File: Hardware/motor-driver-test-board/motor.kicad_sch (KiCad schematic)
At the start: 8 parts, among them J1 Conn_01x11, J2 Conn_01x08, Q1 MMBF170, Q2 MMBF170, Q3 MMBF170, Q4 MMBF170, Q5 MMBF170, Q6 MMBF170

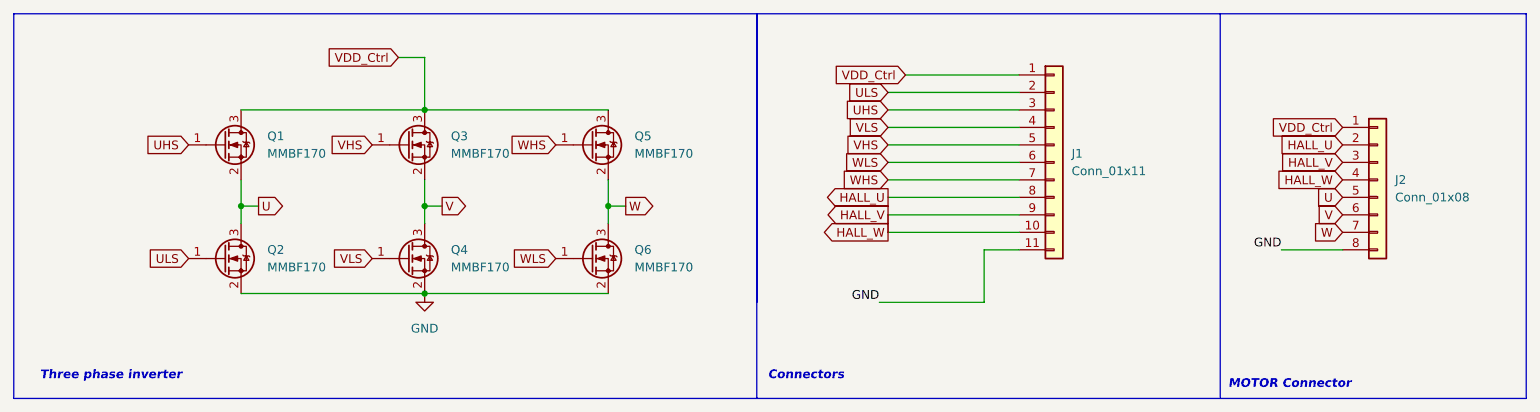
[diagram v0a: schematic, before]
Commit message: PCB REV 1.0
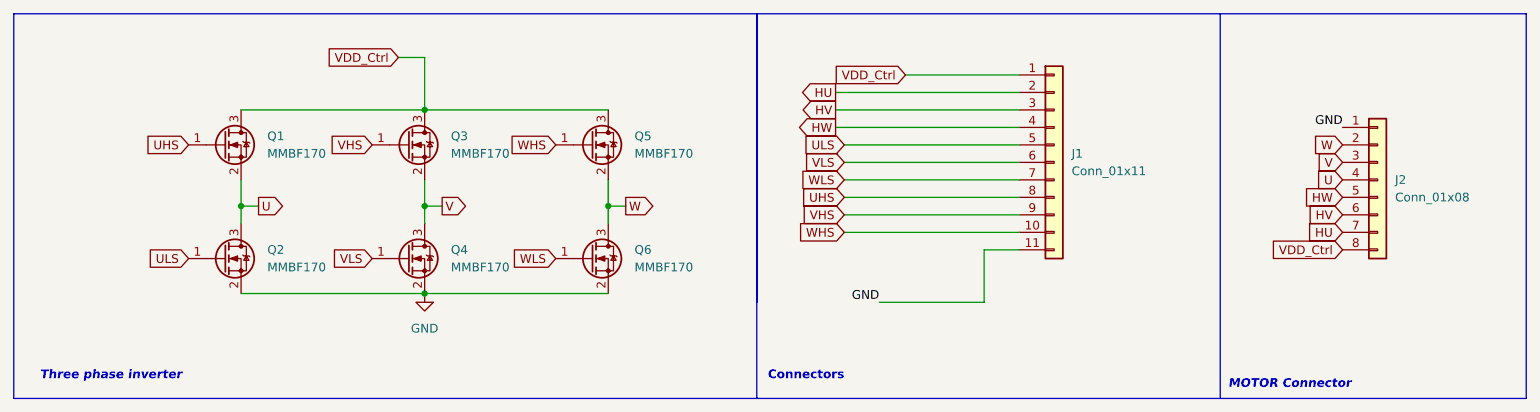
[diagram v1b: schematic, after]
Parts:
- J1: footprint (none) -> Connector_PinHeader_2.54mm:PinHeader_1x11_P2.54mm_Vertical
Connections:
- net GND: now also J2.1 (Pin_1); no longer J2.8 (Pin_8)
- net U: now also J2.4 (Pin_4); no longer J2.5 (Pin_5)
- net UHS: now also J1.8 (Pin_8); no longer J1.3 (Pin_3)
- net ULS: now also J1.5 (Pin_5); no longer J1.2 (Pin_2)
- net V: now also J2.3 (Pin_3); no longer J2.6 (Pin_6)
- net VDD_Ctrl: now also J2.8 (Pin_8); no longer J2.1 (Pin_1)
- net VHS: now also J1.9 (Pin_9); no longer J1.5 (Pin_5)
- net VLS: now also J1.6 (Pin_6); no longer J1.4 (Pin_4)
- net W: now also J2.2 (Pin_2); no longer J2.7 (Pin_7)
- net WHS: now also J1.10 (Pin_10); no longer J1.7 (Pin_7)
- net WLS: now also J1.7 (Pin_7); no longer J1.6 (Pin_6)
- removed net HALL_U: J1.8 (Pin_8), J2.2 (Pin_2)
- removed net HALL_V: J1.10 (Pin_10), J1.9 (Pin_9), J2.3 (Pin_3), J2.4 (Pin_4)
- new net HU: J1.2 (Pin_2), J2.7 (Pin_7)
- new net HV: J1.3 (Pin_3), J2.6 (Pin_6)
- new net HW: J1.4 (Pin_4), J2.5 (Pin_5)
